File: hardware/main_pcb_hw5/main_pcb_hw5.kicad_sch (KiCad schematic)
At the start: 17 parts, among them J1 Barrel_Jack(+12V), J2 5V Buck (MPM3610), J3 3.3V Buck (MPM3610), J4 CART SLOT TOP ROW, J5 CART SLOT BOTTOM ROW, J6 Conn_01x07, J7 EXP1, J8 EXP2, SW1 POWER

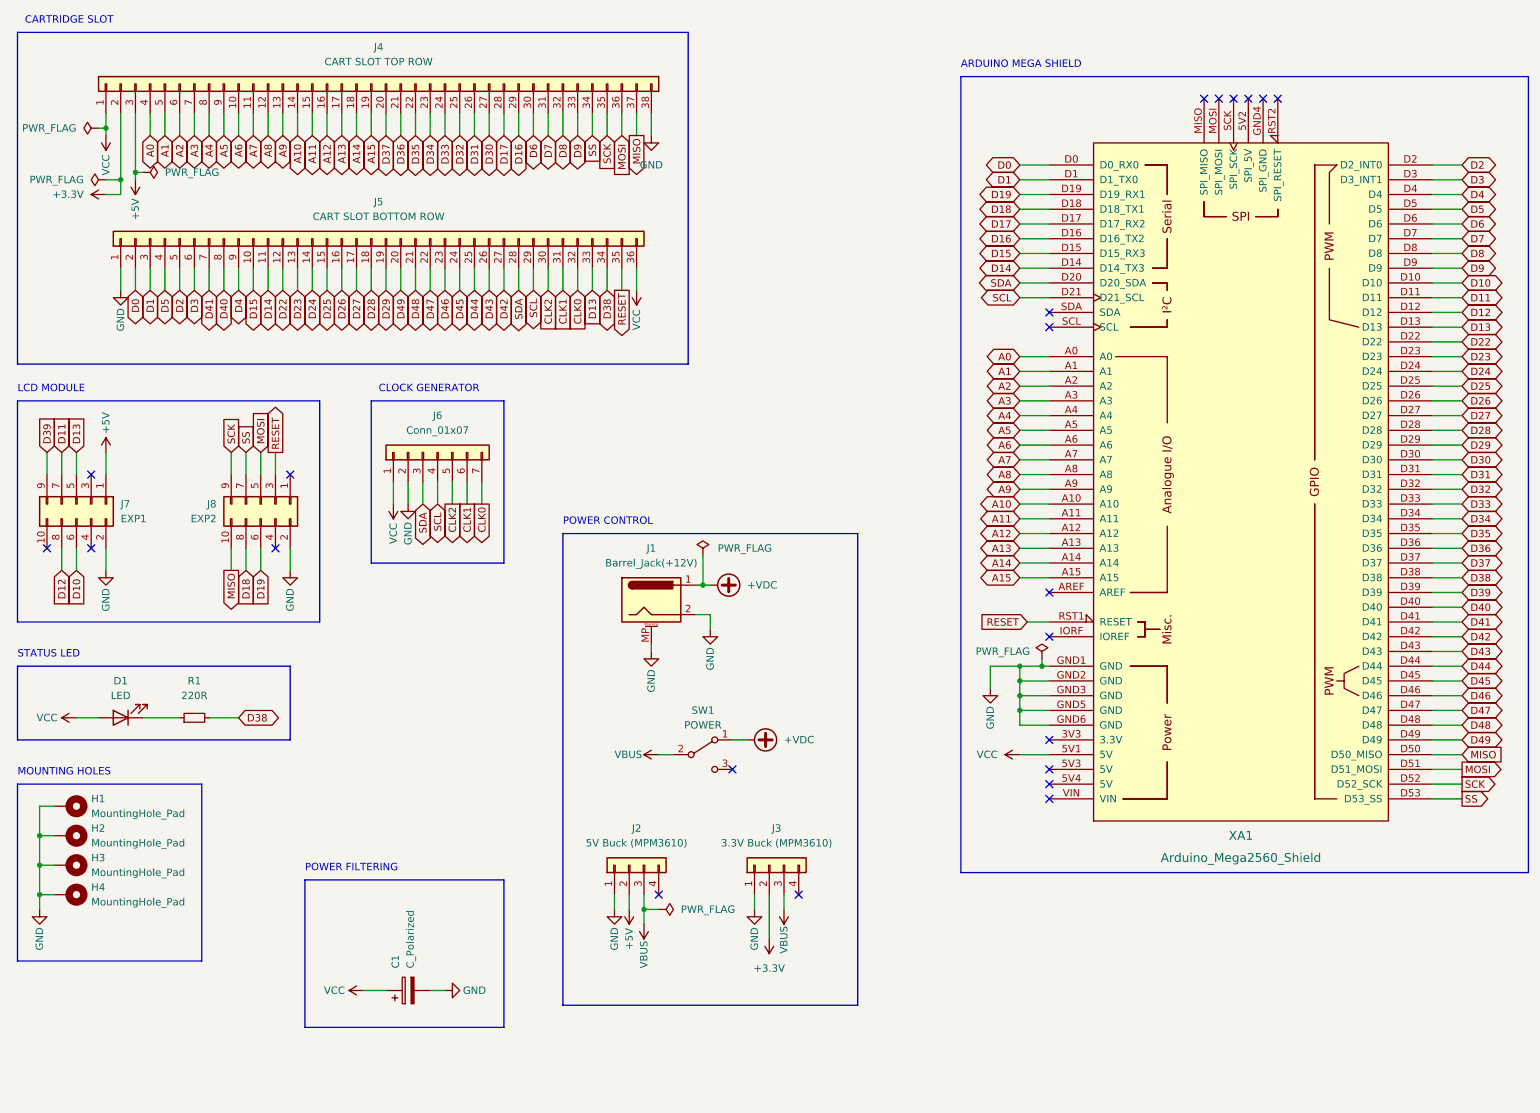
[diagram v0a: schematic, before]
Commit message: export schematic pdf
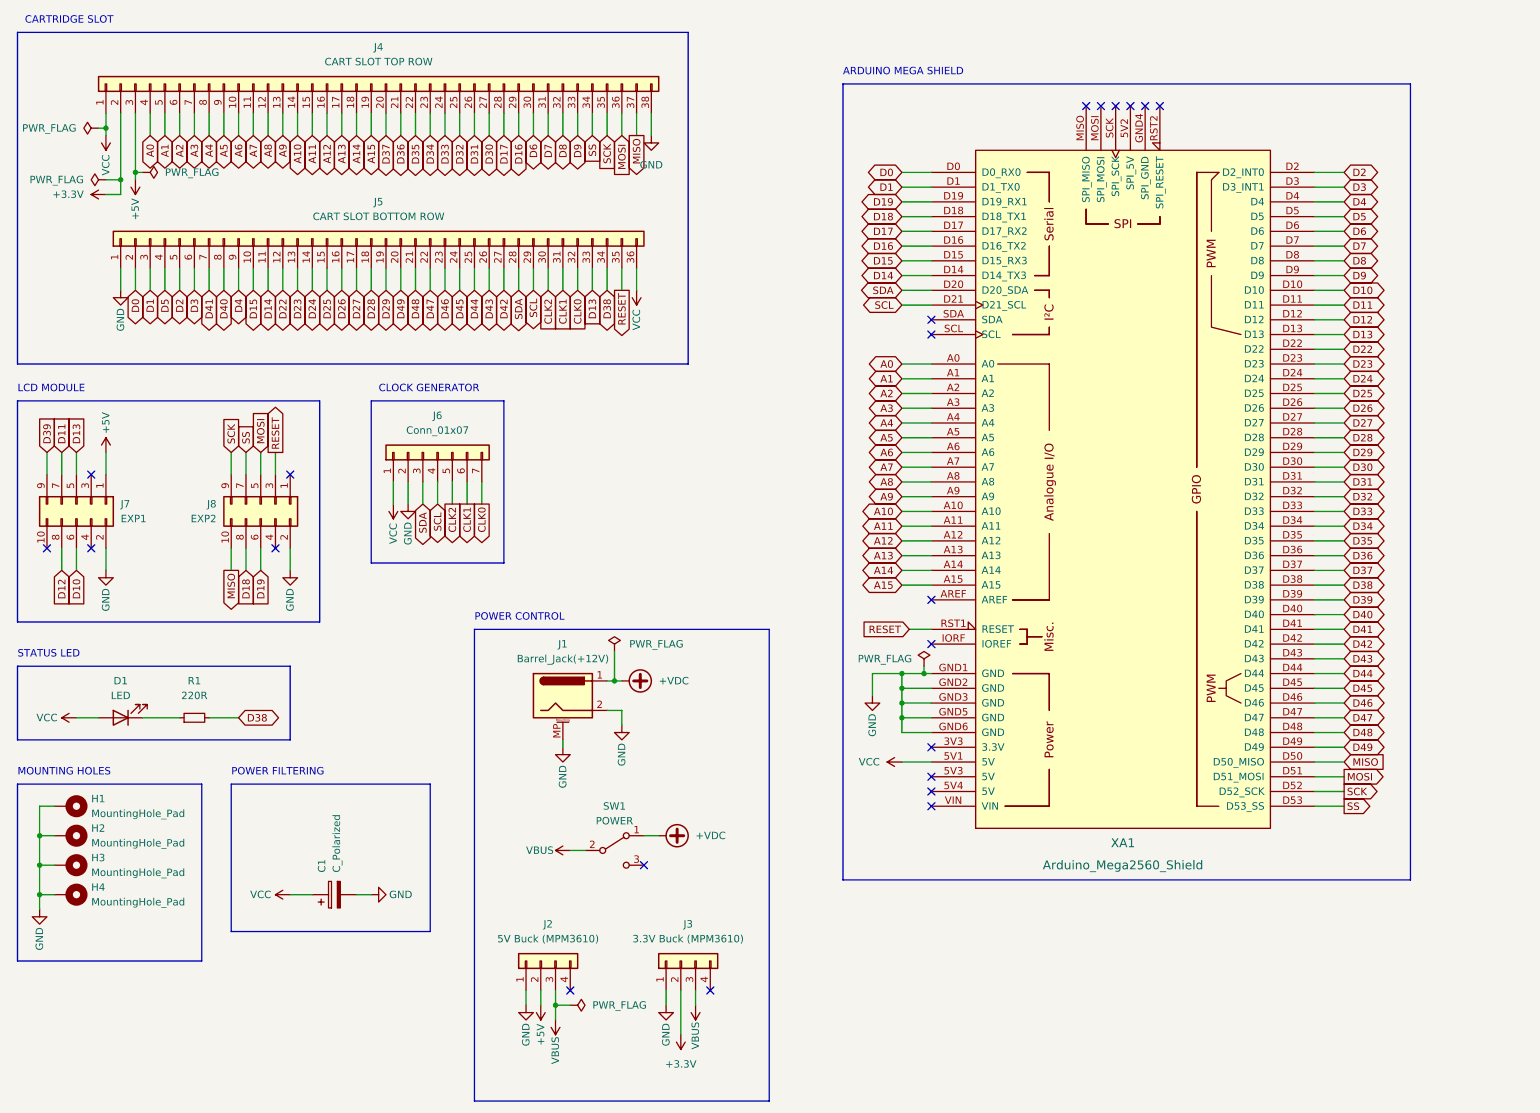
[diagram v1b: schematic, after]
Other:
- title: OSCR HW5 -> OSCR Shield
- moved on the sheet: C1, J1, J2, J3, SW1, XA1
